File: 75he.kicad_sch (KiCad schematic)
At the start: 0 parts

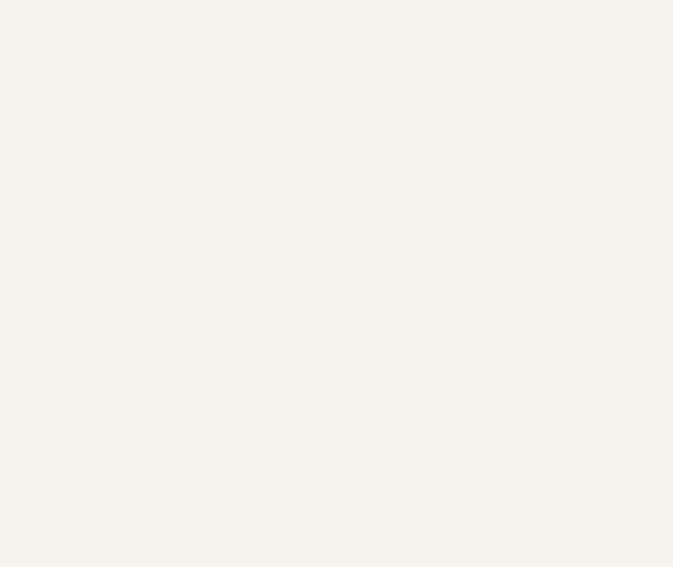
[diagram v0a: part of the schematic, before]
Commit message: fixes & doc
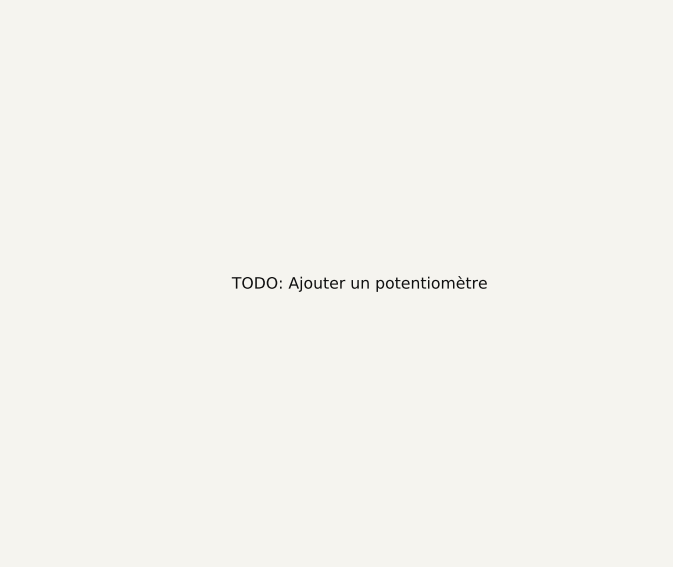
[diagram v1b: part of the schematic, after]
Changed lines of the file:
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@@
+		)
+	)
+	(label "TODO: Ajouter un potentiomètre"
+		(at 231.14 119.38 0)
+		(effects
+			(font
+				(size 1.27 1.27)
+			)
+			(justify left bottom)
 		)
 	)
